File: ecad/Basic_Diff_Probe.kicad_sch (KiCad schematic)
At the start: 37 parts, among them J1 9V Battery Input, J2 To Scope, J3 Differential Input, SW1 EG2209A, U2 LMC6484AIN

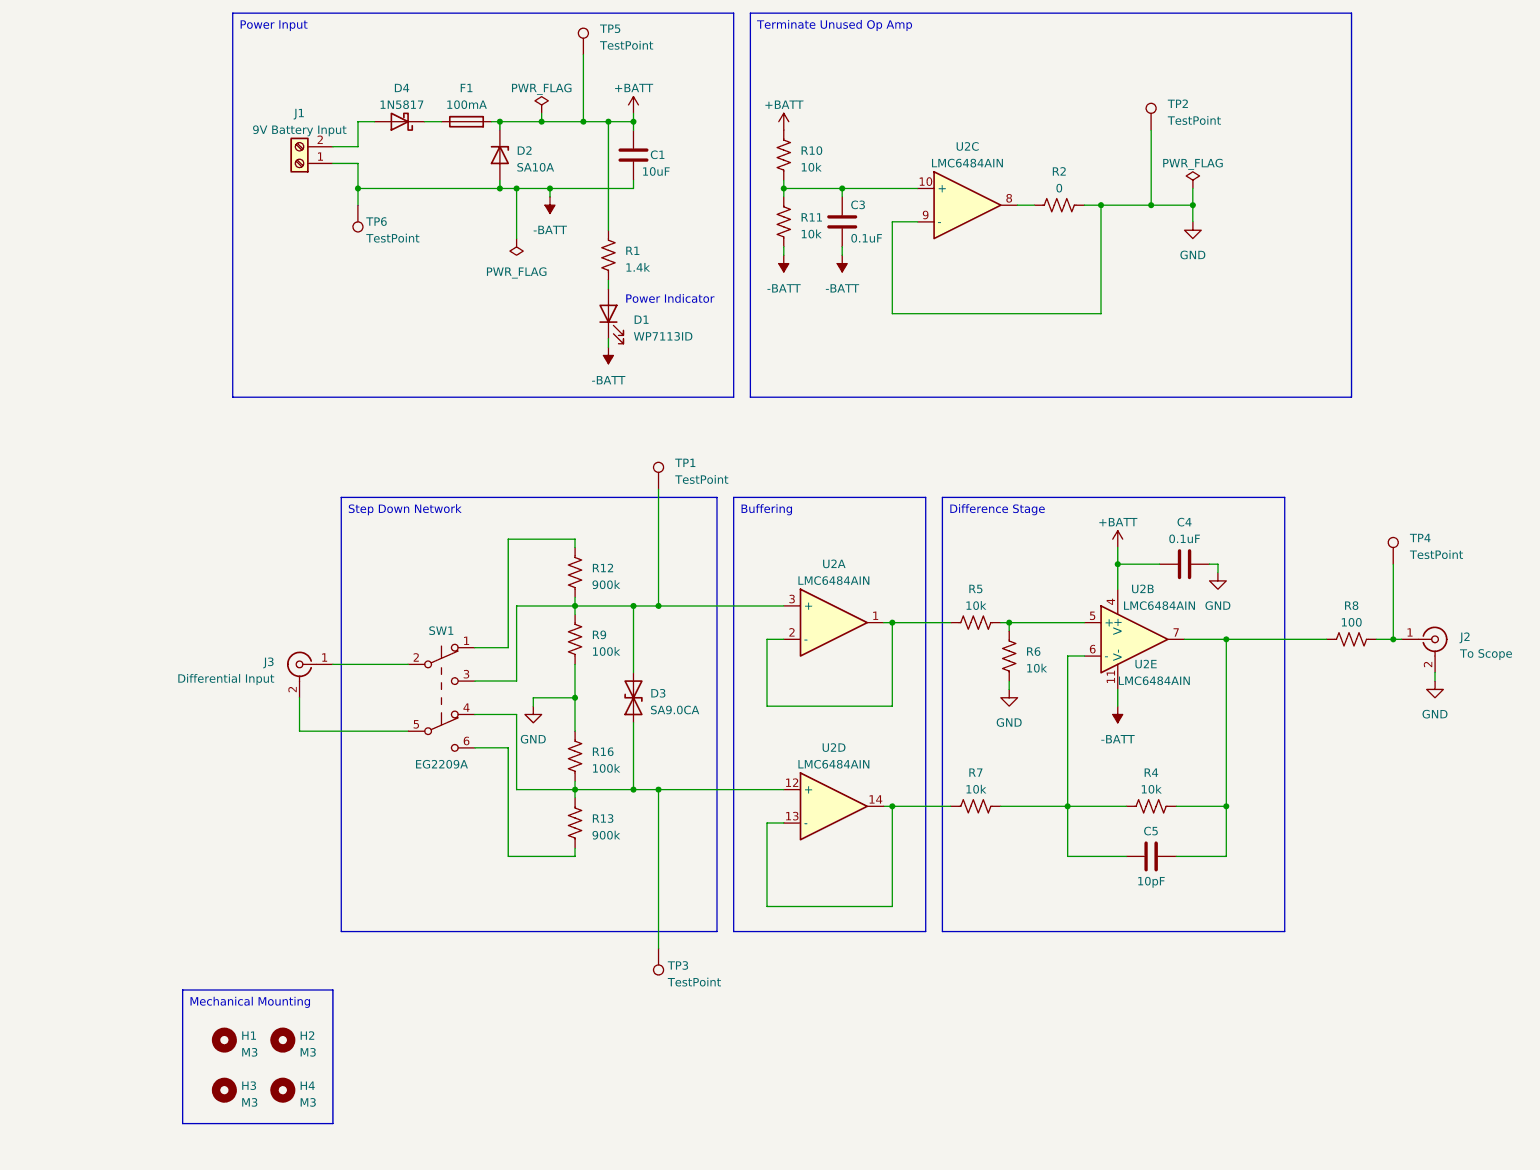
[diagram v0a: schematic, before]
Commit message: outputs
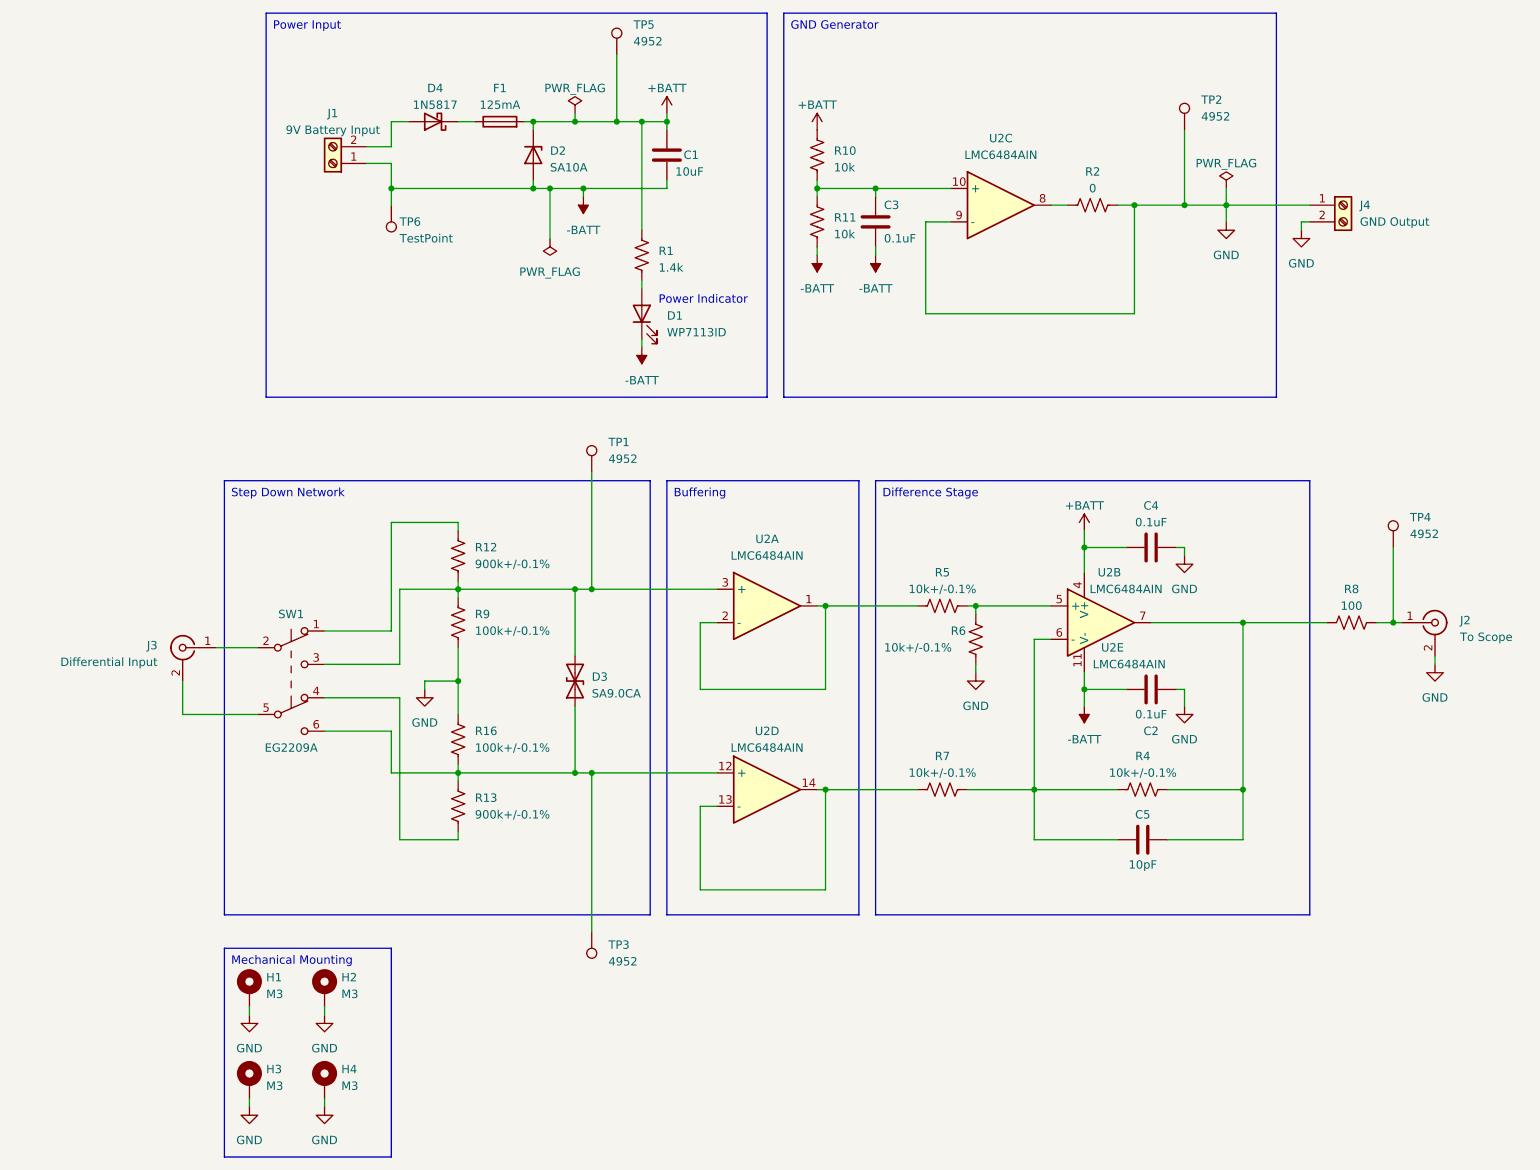
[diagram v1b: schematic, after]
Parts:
- removed H1, H2, H3, H4: M3, MountingHole:MountingHole_3.2mm_M3, symbol Mechanical:MountingHole
- added C2: 0.1uF, Capacitor_THT:C_Disc_D6.0mm_W2.5mm_P5.00mm, symbol Device:C
- added H1, H2, H3, H4: M3, MountingHole:MountingHole_3.2mm_M3_Pad_Via, symbol Mechanical:MountingHole_Pad
- added J4: GND Output, TerminalBlock_Phoenix:TerminalBlock_Phoenix_MKDS-1,5-2-5.08_1x02_P5.08mm_Horizontal, symbol Connector:Screw_Terminal_01x02
- F1: value 100mA -> 125mA
- J2, J3: footprint (none) -> Connector_Coaxial:BNC_Amphenol_031-5539_Vertical
- R12, R13: value 900k -> 900k+/-0.1%
- R16, R9: value 100k -> 100k+/-0.1%
- R4, R5, R6, R7: value 10k -> 10k+/-0.1%
- SW1: footprint (none) -> Diff_Probe_Parts:SW_EG2209A
- TP1, TP2, TP3, TP4, TP5: value TestPoint -> 4952; footprint TestPoint:TestPoint_Keystone_5000-5004_Miniature -> TestPoint:TestPoint_THTPad_2.5x2.5mm_Drill1.2mm
- TP6: footprint TestPoint:TestPoint_Keystone_5000-5004_Miniature -> TestPoint:TestPoint_THTPad_2.5x2.5mm_Drill1.2mm
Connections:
- net +BATT: now also C4.2; no longer C4.1
- net -BATT: now also C2.2
- net GND: now also C4.1, C2.1, H1.1, H2.1, H3.1, H4.1, J4.1 (Pin_1), J4.2 (Pin_2); no longer C4.2
- net at D3.1 (A1), R13.1, R16.2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: now also SW1.6 (C); no longer SW1.4 (A)
- net at R13.2: now also SW1.4 (A); no longer SW1.6 (C)
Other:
- moved on the sheet: C1, C3, C4, C5, D1, D2, D3, D4, F1, J1, J2, J3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
